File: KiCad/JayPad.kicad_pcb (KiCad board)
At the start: 2 copper layers, 107.2 x 54.8 mm, 9 parts, among them SW1 SW_Push, SW2 SW_Push, SW3 SW_Push, SW4 SW_Push, SW5 SW_Push, SW6 SW_Push, U1 XIAO-RP2040-DIP

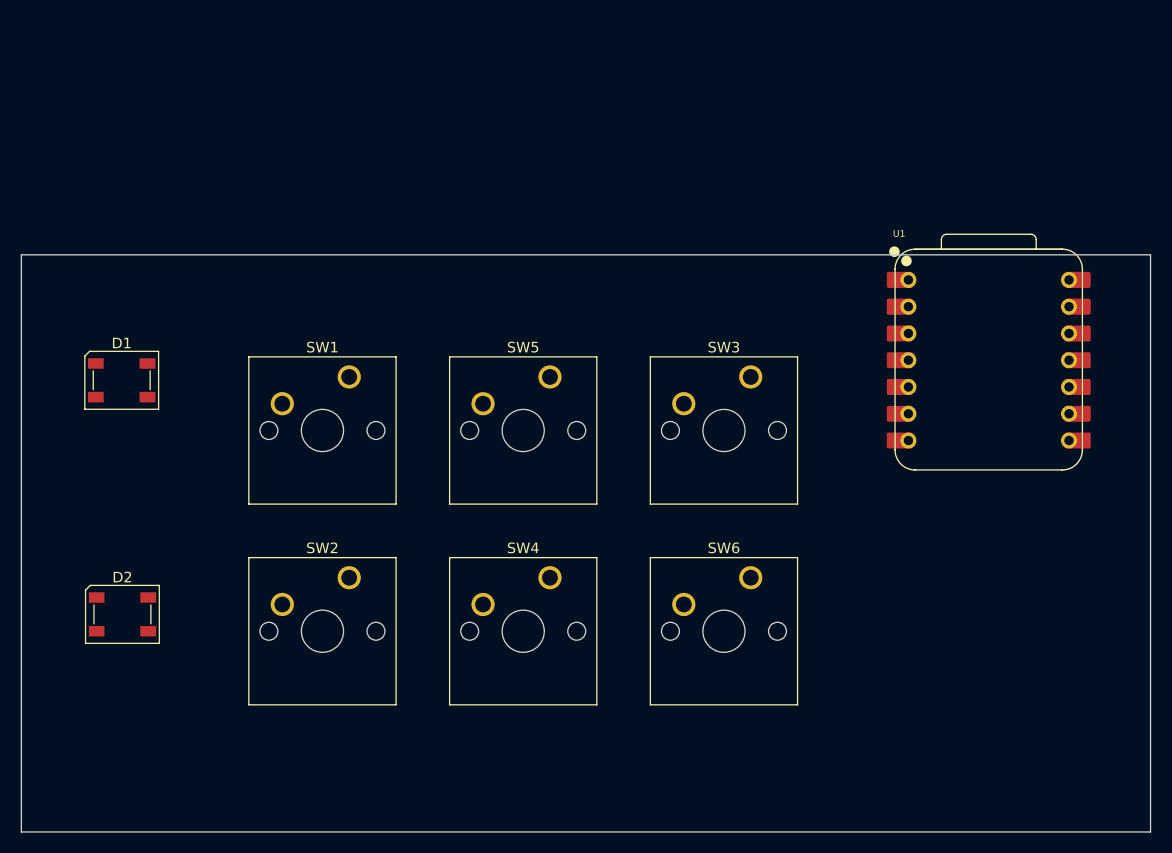
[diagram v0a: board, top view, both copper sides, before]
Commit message: Finished Routing PCB!
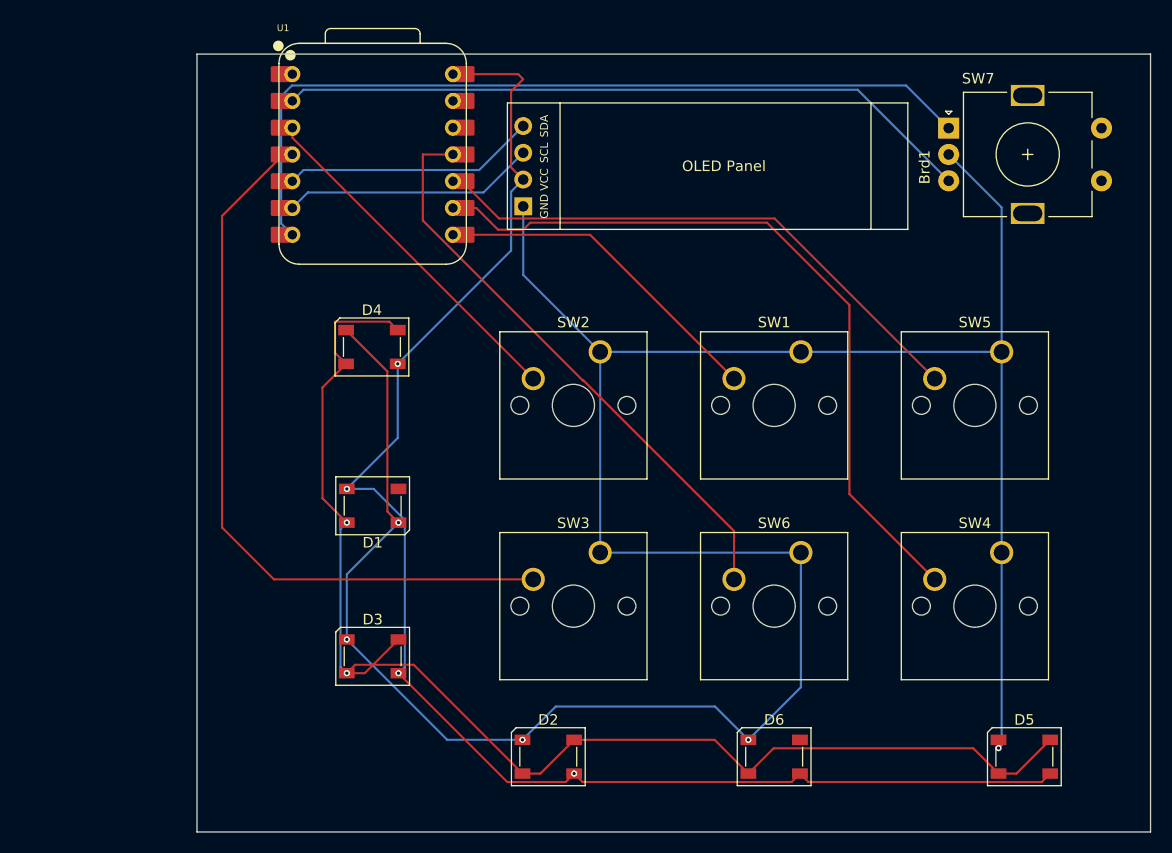
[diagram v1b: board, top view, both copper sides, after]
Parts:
- added Brd1: SSD1306, KiCad-SSD1306-0.91-OLED-4pin-128x32.pretty-master:SSD1306-0.91-OLED-4pin-128x32, F.Cu at (205.6, 42.8)
- added D3: SK6812, LED_SMD:LED_SK6812_PLCC4_5.0x5.0mm_P3.2mm, F.Cu at (154.8, 83.3)
- added D4: SK6812, LED_SMD:LED_SK6812_PLCC4_5.0x5.0mm_P3.2mm, F.Cu at (154.7, 54.0)
- added D5: SK6812, LED_SMD:LED_SK6812_PLCC4_5.0x5.0mm_P3.2mm, F.Cu at (216.6, 92.9)
- added D6: SK6812, LED_SMD:LED_SK6812_PLCC4_5.0x5.0mm_P3.2mm, F.Cu at (192.9, 92.9)
- added SW7: RotaryEncoder, Rotary_Encoder:RotaryEncoder_Alps_EC11E-Switch_Vertical_H20mm, F.Cu at (209.4, 33.2)
- moved U1 61.6 mm to (154.8, 35.7)
- moved SW4 42.9 mm to (214.5, 73.5)
- moved SW5 42.9 mm to (214.5, 54.5)
- moved SW1 42.9 mm to (195.4, 54.5)
- moved D2 42.6 mm to (171.4, 92.9)
- moved SW2 32.0 mm to (176.4, 54.5)
- moved D1 26.6 mm to (154.8, 69.1), turned to 180 degrees
- moved SW3 22.0 mm to (176.4, 73.5)
- moved SW6 5.32 mm to (195.4, 73.5)
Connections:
- D2 pad 4: unconnected-(D2-DOUT-Pad4) -> Net-(D1-DOUT)
- SW4 pad 2: Net-(U1-GPIO3/MOSI) -> Net-(U1-GPIO2/SCK)
- SW6 pad 2: Net-(U1-GPIO2/SCK) -> Net-(U1-GPIO3/MOSI)
- U1 pad 1: unconnected-(U1-GPIO26/ADC0/A0-Pad1) -> Net-(D1-DIN)
- U1 pad 13: unconnected-(U1-GND-Pad13) -> GND
- U1 pad 14: unconnected-(U1-VBUS-Pad14) -> +5V
- U1 pad 2: unconnected-(U1-GPIO27/ADC1/A1-Pad2) -> Net-(U1-GPIO27/ADC1/A1)
- U1 pad 5: Net-(D1-DIN) -> Net-(Brd1-SDA)
- U1 pad 6: unconnected-(U1-GPIO7/SCL-Pad6) -> Net-(Brd1-SCL)
- U1 pad 7: unconnected-(U1-GPIO0/TX-Pad7) -> Net-(U1-GPIO0/TX)
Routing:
- net GND: track 0.00 -> 249.5 mm, vias 0 -> 6
- net +5V: track 0.00 -> 142.1 mm, vias 0 -> 4
- net Net-(D1-DOUT): track 0.00 -> 126.0 mm, vias 0 -> 2
- net Net-(U1-GPIO0/TX): track 0.00 -> 79.0 mm
- net Net-(U1-GPIO2/SCK): track 0.00 -> 70.5 mm
- net Net-(U1-GPIO29/ADC3/A3): track 0.00 -> 70.2 mm
- net Net-(U1-GPIO27/ADC1/A1): track 0.00 -> 66.3 mm
- net Net-(U1-GPIO3/MOSI): track 0.00 -> 55.4 mm
- net Net-(U1-GPIO4/MISO): track 0.00 -> 52.6 mm
- net Net-(U1-GPIO28/ADC2/A2): track 0.00 -> 33.3 mm
- net Net-(U1-GPIO1/RX): track 0.00 -> 31.5 mm
- net Net-(Brd1-SDA): track 0.00 -> 24.1 mm, vias 0 -> 1
- net Net-(Brd1-SCL): track 0.00 -> 24.1 mm
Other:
- board size 107.2 x 54.8 mm -> 90.5 x 73.8 mm
